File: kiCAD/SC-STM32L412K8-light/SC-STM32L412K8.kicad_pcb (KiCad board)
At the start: 2 copper layers, 31.6 x 15.1 mm, 66 parts, among them J1 usb, J10 Buzzer, J11 Vibro, J12 +3v, J13 +vibro, J2 +29.6 SiPM, J3 TxD (20), J4 RxD (19), J5 SWDIO, J6 SWCLK, J7 +BAT, J8 SiPM-, J9 BT Status, Q1 IRLML6344, Q2 IRLML6344, SW1 power, U2 AP3015KTR, U3 MCP73831, U4 TLV3201AIDBVT, U5 MCP1700-3002E

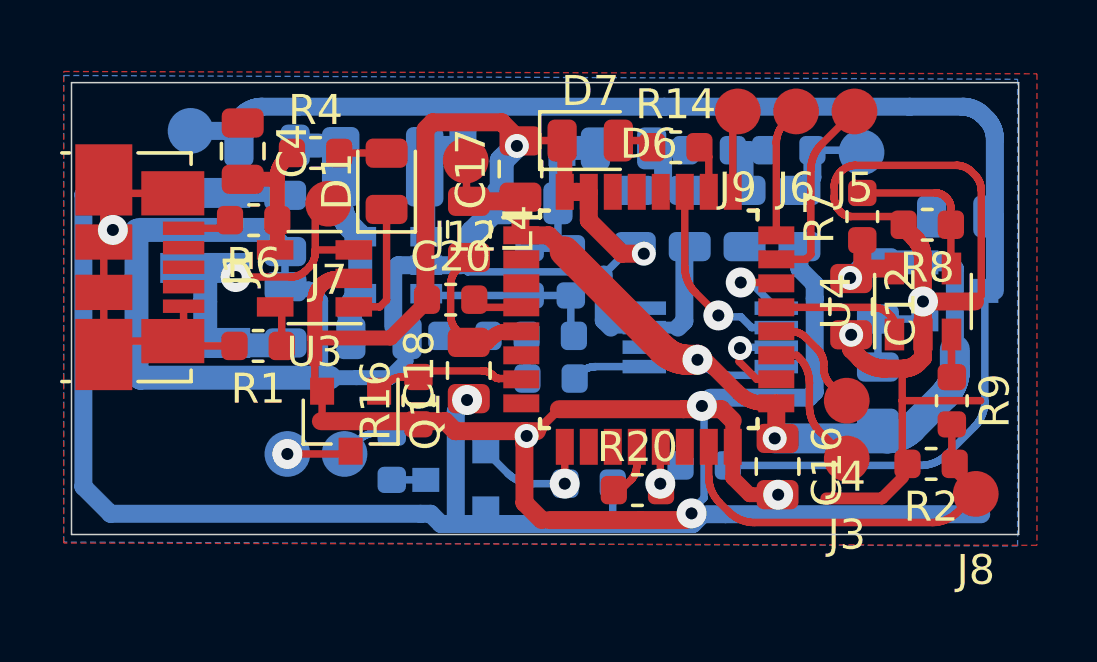
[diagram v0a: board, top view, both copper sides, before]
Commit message: modified:   kiCAD/SC-STM32L412K8-light/SC-STM32L412K8.kicad_pcb 	modified:   kiCAD/SC-STM32L412K8-light/SC-STM32L412K8.kicad_pcb-bak
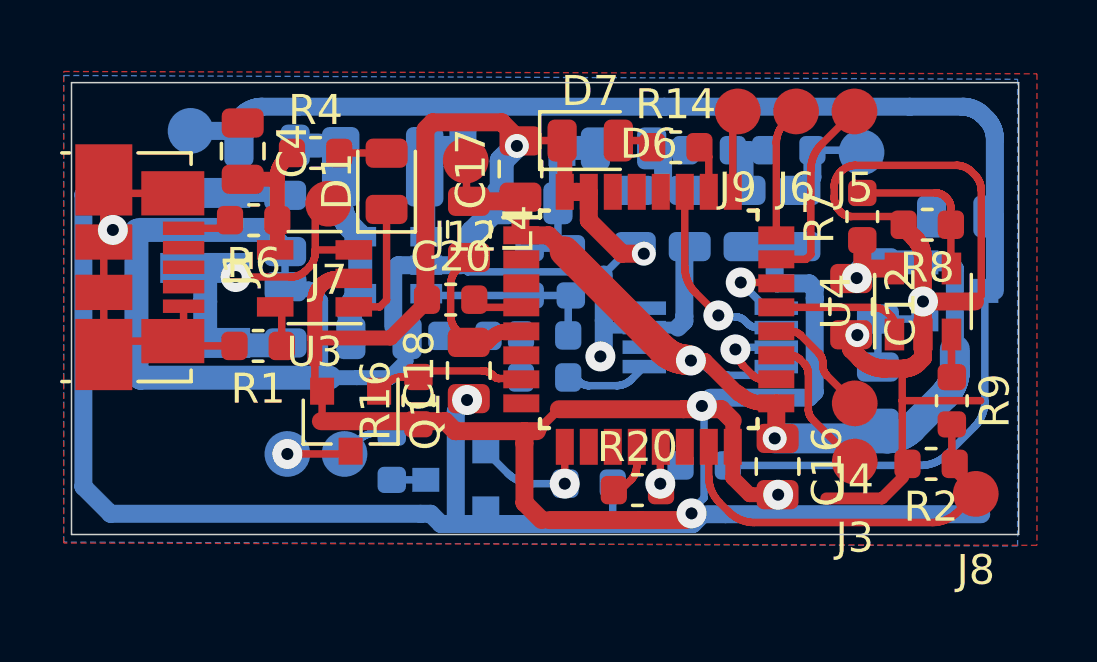
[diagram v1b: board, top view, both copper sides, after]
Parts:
- moved J3 0.28 mm to (53.6, 65.5)
- moved J4 0.28 mm to (53.6, 63.6)
- moved R17 0.22 mm to (43.2, 62.7)
- moved R3 0.19 mm to (43.2, 61.3)
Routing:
- net GND: track 208.9 -> 212.6 mm
